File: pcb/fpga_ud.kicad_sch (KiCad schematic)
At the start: 1 part

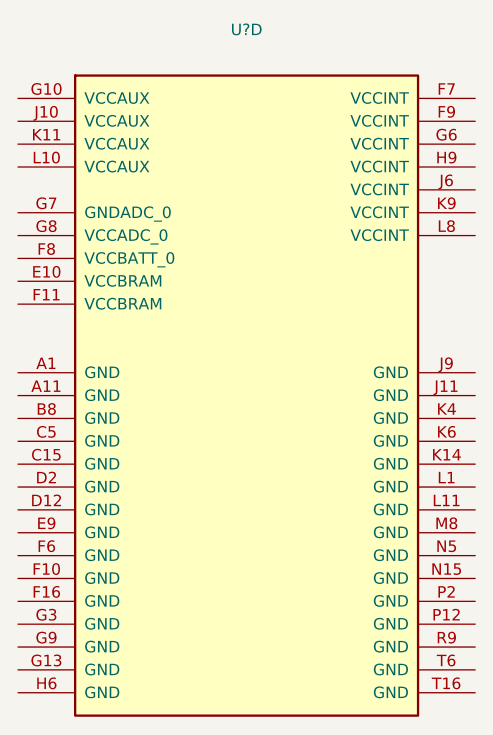
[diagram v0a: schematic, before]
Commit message: kicad said I needed to save
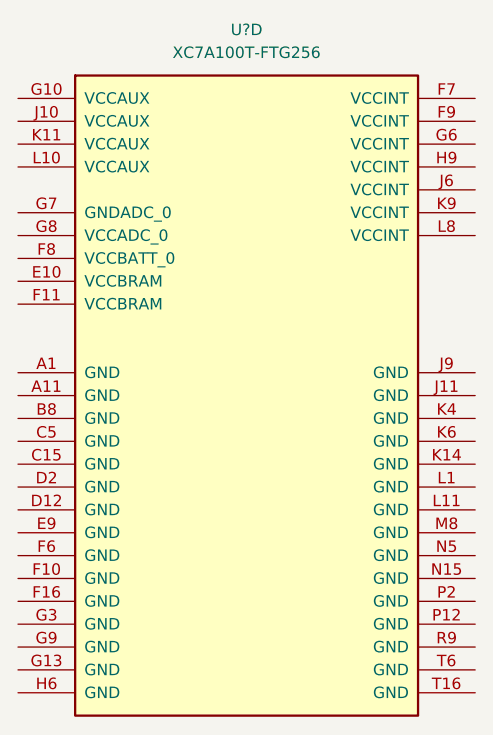
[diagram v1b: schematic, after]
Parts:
- U?: value (none) -> XC7A100T-FTG256
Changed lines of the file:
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@@
     (in_bom yes) (on_board yes) (fields_autoplaced)
     (property "Reference" "U?" (id 0) (at 96.52 44.45 0))
-    (property "Value" "" (id 1) (at 96.52 46.99 0))
+    (property "Value" "XC7A100T-FTG256" (id 1) (at 96.52 46.99 0))
     (property "Footprint" "" (id 2) (at 96.52 85.09 0)
       (effects (font (size 1.27 1.27)) hide)
